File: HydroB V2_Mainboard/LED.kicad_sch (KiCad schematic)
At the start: 9 parts, among them J2 Conn_01x02_Pin, J4 Conn_01x02_Pin, J8 LCD, Q1 S8050, Q2 S8050

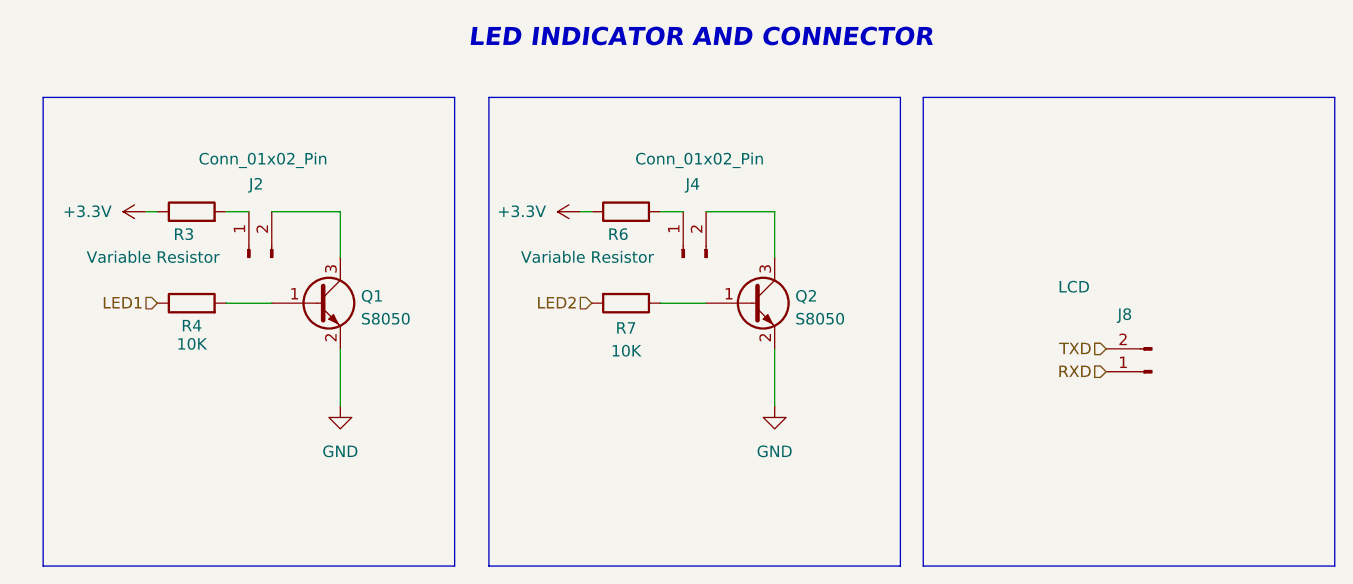
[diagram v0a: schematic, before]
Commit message: PCB placement and ERC
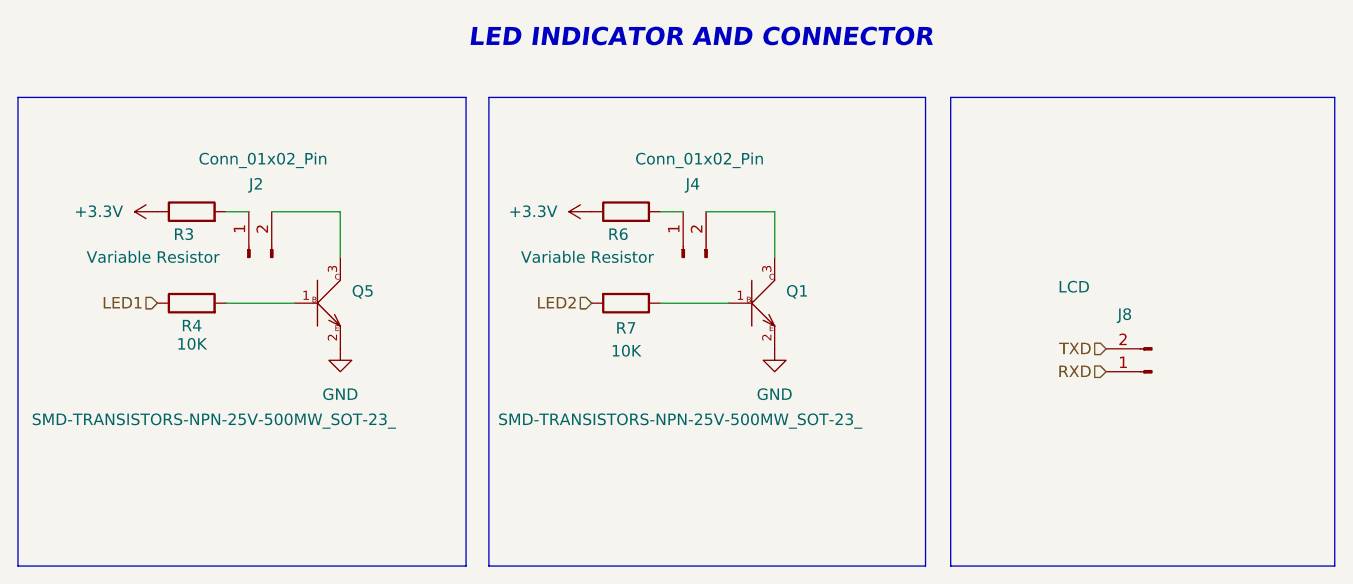
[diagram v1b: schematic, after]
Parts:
- removed Q1, Q2: S8050, Package_TO_SOT_SMD:SOT-23, symbol Transistor_BJT:S8050
- added Q1, Q5: SMD-TRANSISTORS-NPN-25V-500MW_SOT-23_, SMD-TRANSISTORS-NPN-25V-500MW_SOT-23_:SOT-23, symbol S8050:SMD-TRANSISTORS-NPN-25V-500MW_SOT-23_
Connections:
- net GND: now also Q1.2, Q5.2
- net at R7.1: now also Q1.1
- net at R4.2: now also Q5.1
- net at J2.2 (Pin_2): now also Q5.3
- net at J4.2 (Pin_2): now also Q1.3
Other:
- company: (none) -> LED Indicator
- title: (none) -> Prak Chilifong
